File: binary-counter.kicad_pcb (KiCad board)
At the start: 2 copper layers, 97 x 52 mm, 33 parts, among them J1 Power, SW1 Clock, SW2 SW_SPDT, SW3 SW_SPDT, U1 NE555P, U17 SM410561K, U18 74HC86, U19 SM410561K, U2 NE555P, U20 74LS248, U21 74LS83, U22 74LS191, U3 74HC00, U4 NE555P

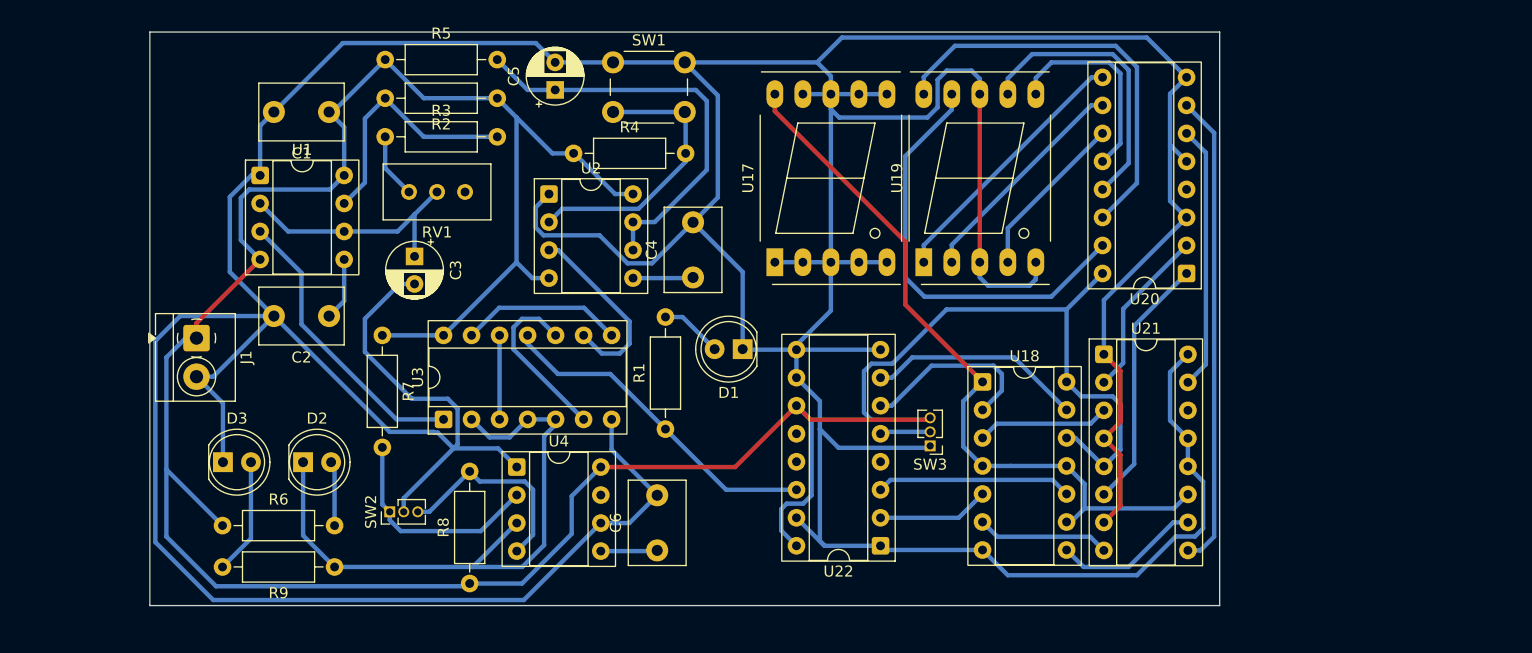
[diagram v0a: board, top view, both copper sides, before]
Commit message: finished
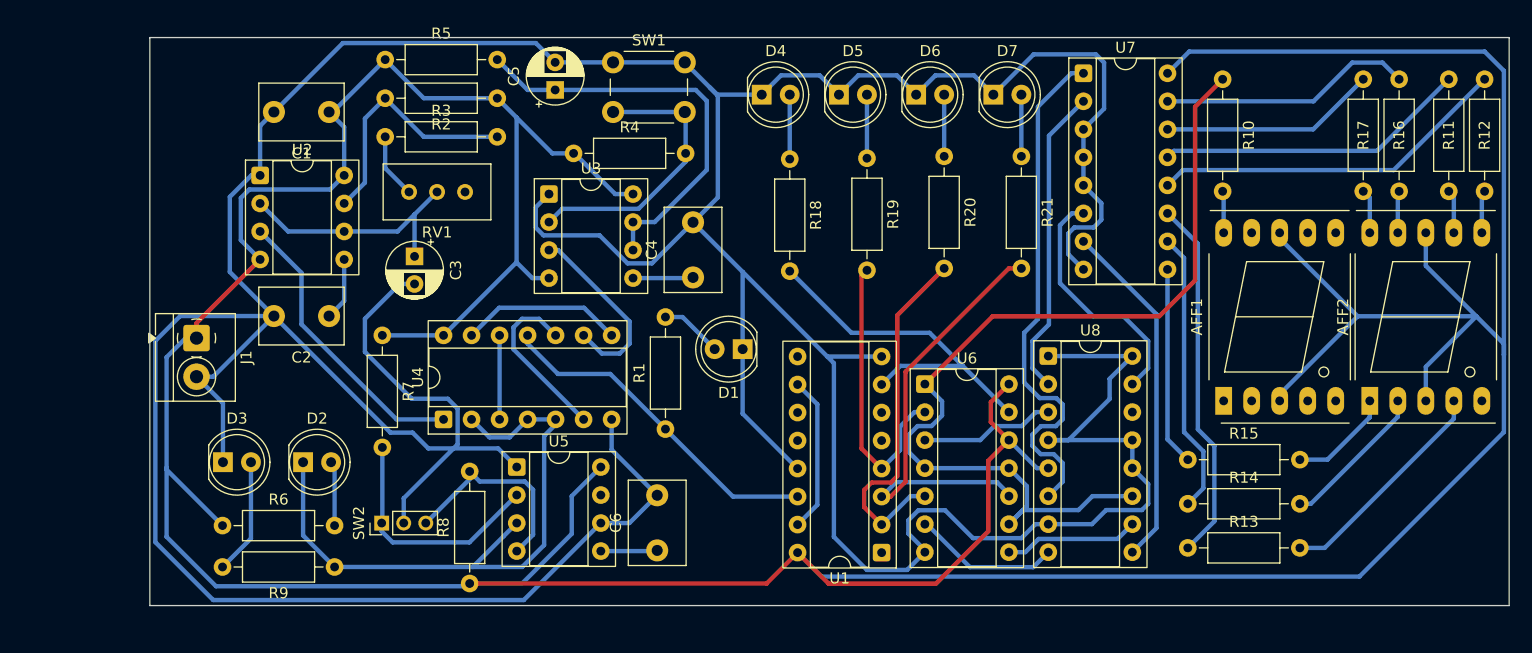
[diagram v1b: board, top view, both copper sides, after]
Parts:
- removed SW3: SW_SPDT, Connector_PinHeader_1.27mm:PinHeader_1x03_P1.27mm_Vertical
- removed U17, U19: SM410561K, Display_7Segment:7SegmentLED_LTS6760_LTS6780
- removed U20: 74LS248, Package_DIP:DIP-16_W7.62mm_Socket
- removed U22: 74LS191, Package_DIP:DIP-16_W7.62mm_Socket
- added AFF1: LTS-6960HR, Display_7Segment:7SegmentLED_LTS6760_LTS6780, F.Cu at (196.1, 102.2)
- added AFF2: LTS-6960HR, Display_7Segment:7SegmentLED_LTS6760_LTS6780, F.Cu at (209.3, 102.2)
- added D4: Red, LED_THT:LED_D5.0mm, F.Cu at (154.2, 74.4)
- added D5: Red, LED_THT:LED_D5.0mm, F.Cu at (161.2, 74.4)
- added D6: Red, LED_THT:LED_D5.0mm, F.Cu at (168.2, 74.4)
- added D7: Red, LED_THT:LED_D5.0mm, F.Cu at (175.2, 74.4)
- added R10: 220 R, Resistor_THT:R_Axial_DIN0207_L6.3mm_D2.5mm_P10.16mm_Horizontal, F.Cu at (196.0, 73.0)
- added R11: 220 R, Resistor_THT:R_Axial_DIN0207_L6.3mm_D2.5mm_P10.16mm_Horizontal, F.Cu at (216.5, 73.0)
- added R12: 220 R, Resistor_THT:R_Axial_DIN0207_L6.3mm_D2.5mm_P10.16mm_Horizontal, F.Cu at (219.8, 73.0)
- added R13: 220 R, Resistor_THT:R_Axial_DIN0207_L6.3mm_D2.5mm_P10.16mm_Horizontal, F.Cu at (192.8, 115.5)
- added R14: 220 R, Resistor_THT:R_Axial_DIN0207_L6.3mm_D2.5mm_P10.16mm_Horizontal, F.Cu at (192.8, 111.5)
- added R15: 220 R, Resistor_THT:R_Axial_DIN0207_L6.3mm_D2.5mm_P10.16mm_Horizontal, F.Cu at (192.8, 107.5)
- added R16: 220 R, Resistor_THT:R_Axial_DIN0207_L6.3mm_D2.5mm_P10.16mm_Horizontal, F.Cu at (212.0, 73.0)
- added R17: 220 R, Resistor_THT:R_Axial_DIN0207_L6.3mm_D2.5mm_P10.16mm_Horizontal, F.Cu at (208.8, 73.0)
- added R18: 220 R, Resistor_THT:R_Axial_DIN0207_L6.3mm_D2.5mm_P10.16mm_Horizontal, F.Cu at (156.8, 80.2)
- added R19: 220 R, Resistor_THT:R_Axial_DIN0207_L6.3mm_D2.5mm_P10.16mm_Horizontal, F.Cu at (163.8, 80.2)
- added R20: 220 R, Resistor_THT:R_Axial_DIN0207_L6.3mm_D2.5mm_P10.16mm_Horizontal, F.Cu at (170.8, 80.0)
- added R21: 220 R, Resistor_THT:R_Axial_DIN0207_L6.3mm_D2.5mm_P10.16mm_Horizontal, F.Cu at (177.8, 80.0)
- added U1: 4017, Package_DIP:DIP-16_W7.62mm_Socket, F.Cu at (165.1, 115.9)
- added U7: 74LS47, Package_DIP:DIP-16_W7.62mm_Socket, F.Cu at (183.4, 72.5)
- SW2: value SW_SPDT -> TIM_MODSEL; footprint Connector_PinHeader_1.27mm:PinHeader_1x03_P1.27mm_Vertical -> Connector_PinHeader_2.00mm:PinHeader_1x03_P2.00mm_Vertical
- moved U6 5.23 mm to (169.0, 100.7)
- moved U8 5.04 mm to (180.2, 98.1)
- moved SW2 1.25 mm to (119.8, 113.2)
- renumbered U1 to U2, U2 to U3, U3 to U4, U4 to U5, U18 to U6, U21 to U8
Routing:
- net +5V: track 280.1 -> 435.3 mm
- net GND: track 567.5 -> 463.3 mm
- net Net-(U19-F): track 38.9 -> 0.00 mm
- net Net-(U19-G): track 37.8 -> 0.00 mm
- net Net-(U7-c): track 0.00 -> 33.1 mm
- net Net-(U7-b): track 0.00 -> 32.7 mm
- net Net-(U7-a): track 0.00 -> 28.4 mm
- net Net-(U7-d): track 0.00 -> 25.7 mm
- net Net-(U19-A): track 25.7 -> 0.00 mm
- net Net-(U7-B): track 23.1 -> 47.8 mm
- net Net-(U19-E): track 24.1 -> 0.00 mm
- net Net-(U7-f): track 0.00 -> 23.1 mm
- net /Display/Q1: track 10.1 -> 32.9 mm
- net /Display/Q0: track 17.8 -> 39.8 mm
- net Net-(U19-D): track 20.5 -> 0.00 mm
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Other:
- board size 97 x 52 mm -> 123.2 x 51.5 mm

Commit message: the end
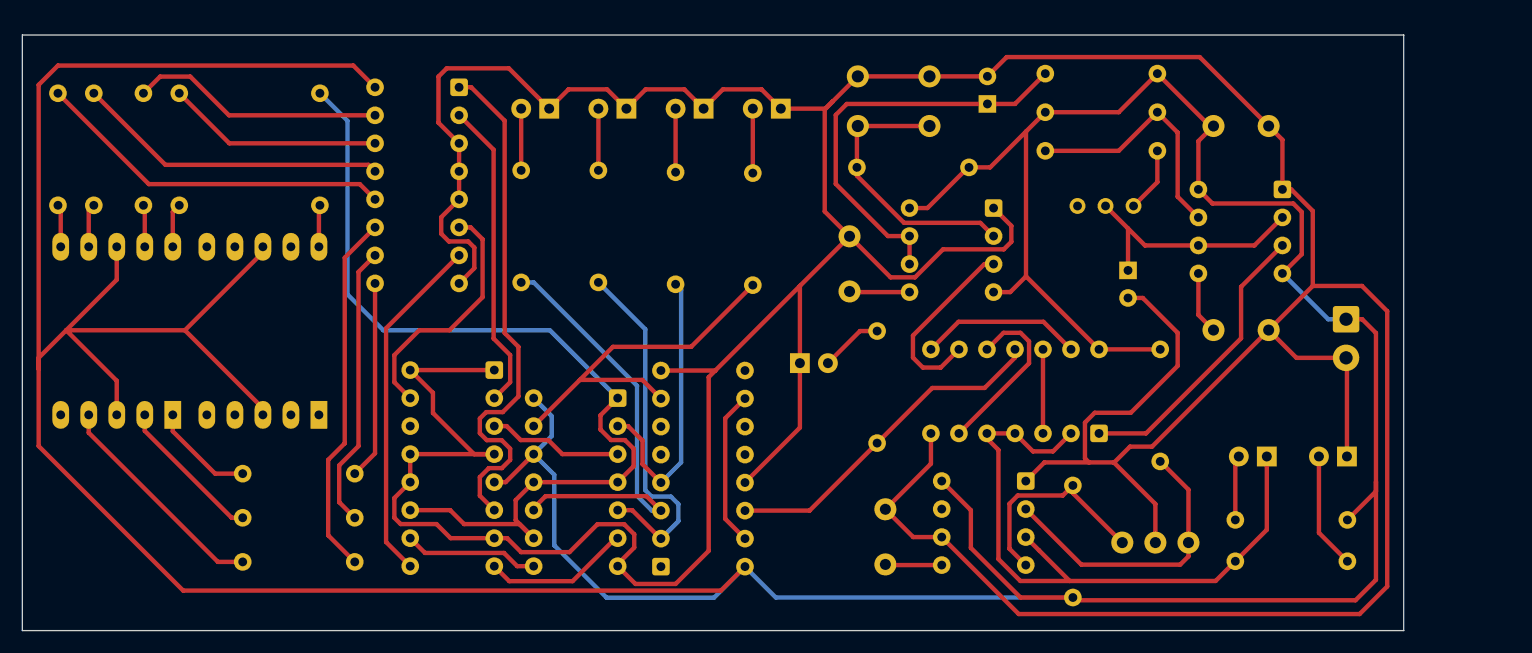
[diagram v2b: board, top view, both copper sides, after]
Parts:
- AFF1, AFF2, C1, C2, C3, C4, C5, C6, D1, D2, D3, D4, D5, D6, D7, J1, R1, R10, R11, R12, R13, R14, R15, R16, R17, R18, R19, R2, R20, R21, R3, R4, R5, R6, R7, R8, R9, RV1, SW1, U1, U2, U3, U4, U5, U6, U7, U8: moved to B.Cu
- SW2: value TIM_MODSEL -> SW_SPDT; footprint Connector_PinHeader_2.00mm:PinHeader_1x03_P2.00mm_Vertical -> Switches:IC-205; moved to B.Cu
- moved R12 129.4 mm to (90.4, 74.3)
- moved R11 122.9 mm to (93.7, 74.3)
- moved R16 113.9 mm to (98.2, 74.3)
- moved AFF2 108.5 mm to (100.8, 103.4)
- moved R17 107.4 mm to (101.4, 74.3)
- moved J1 104.2 mm to (207.2, 94.8)
- moved R6 102.0 mm to (207.3, 113.0), turned to 180 degrees
- moved D3 101.9 mm to (207.3, 107.2), turned to 180 degrees
- moved U2 92.7 mm to (201.4, 83.0), turned to 180 degrees
- moved D2 87.4 mm to (200.0, 107.2), turned to 180 degrees
- moved AFF1 82.0 mm to (114.1, 103.4)
- moved R10 81.9 mm to (114.2, 74.3)
- moved R9 81.7 mm to (197.1, 116.7), turned to 0 degrees
- moved C1 80.2 mm to (195.2, 77.2), turned to 0 degrees
- moved C2 80.2 mm to (195.2, 95.8), turned to 0 degrees
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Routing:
- net Net-(SW2-A): track 22.1 -> 26.8 mm
- net Net-(D2-K): track 56.9 -> 60.1 mm
- net GND: track 463.3 -> 464.6 mm
- net Net-(SW2-C): track 18.9 -> 19.6 mm
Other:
- board size 123.2 x 51.5 mm -> 125.2 x 54 mm
